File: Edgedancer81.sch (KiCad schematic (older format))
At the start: 30 parts

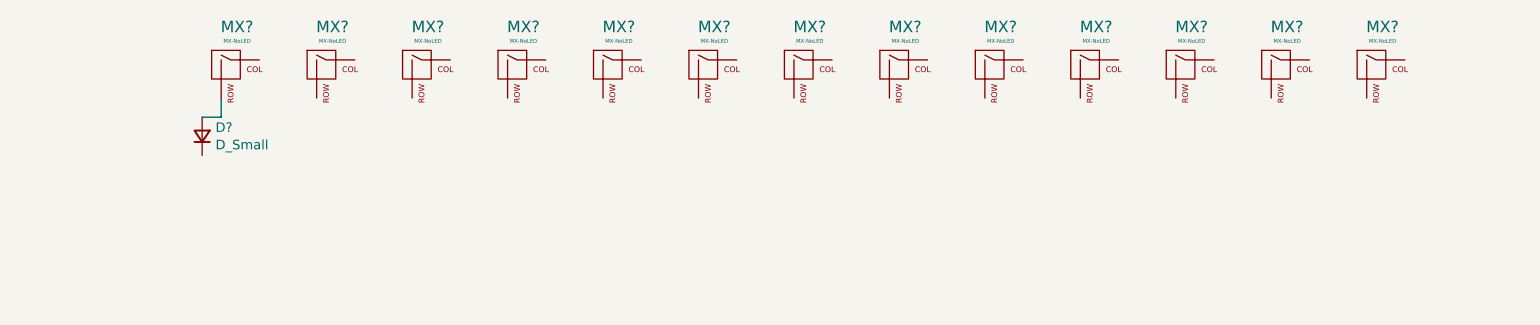
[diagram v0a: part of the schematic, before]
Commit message: more wires
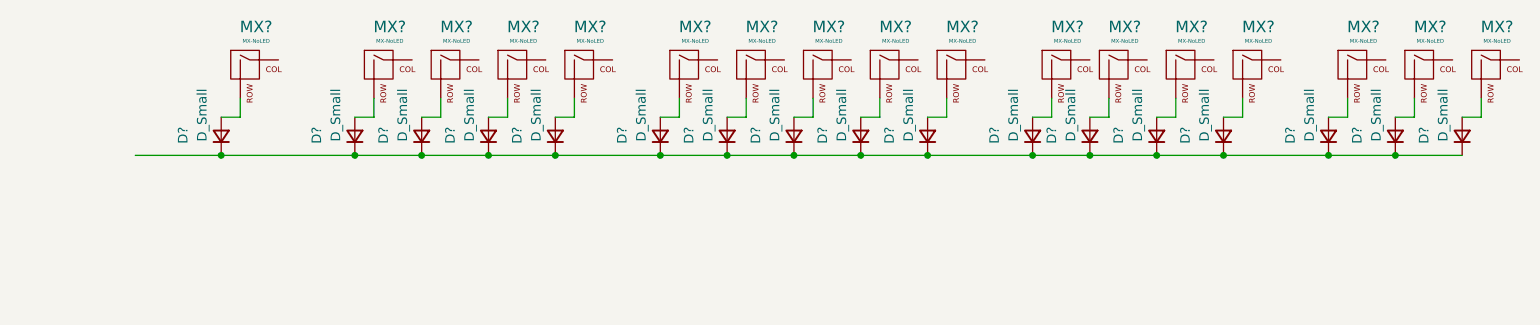
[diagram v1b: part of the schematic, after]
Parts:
- added D? (x16): D_Small, symbol Device:D_Small
- added MX? (x4): MX-NoLED, symbol MX_Alps_Hybrid:MX-NoLED
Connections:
- net at D?.1 (K): now also D?.1 (K), D?.1 (K), D?.1 (K), D?.1 (K), D?.1 (K), D?.1 (K), D?.1 (K), D?.1 (K), D?.1 (K), D?.1 (K), D?.1 (K), D?.1 (K), D?.1 (K), D?.1 (K), D?.1 (K), D?.1 (K)
- net at MX?.2 (ROW): now also D?.2 (A) (x12)
- new net: D?.2 (A), MX?.2 (ROW) (x4)
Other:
- moved on the sheet: D?, MX?
